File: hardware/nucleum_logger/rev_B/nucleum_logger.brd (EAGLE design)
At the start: 34.9 x 73 mm, 16 parts, among them J1 DM3AT-SF-PEJM5, J2 AA_BAT_PACKSMD, J3 SQUALL_HEADER_BASE, Q1 NX3008PBK, U1 NUCLEUM

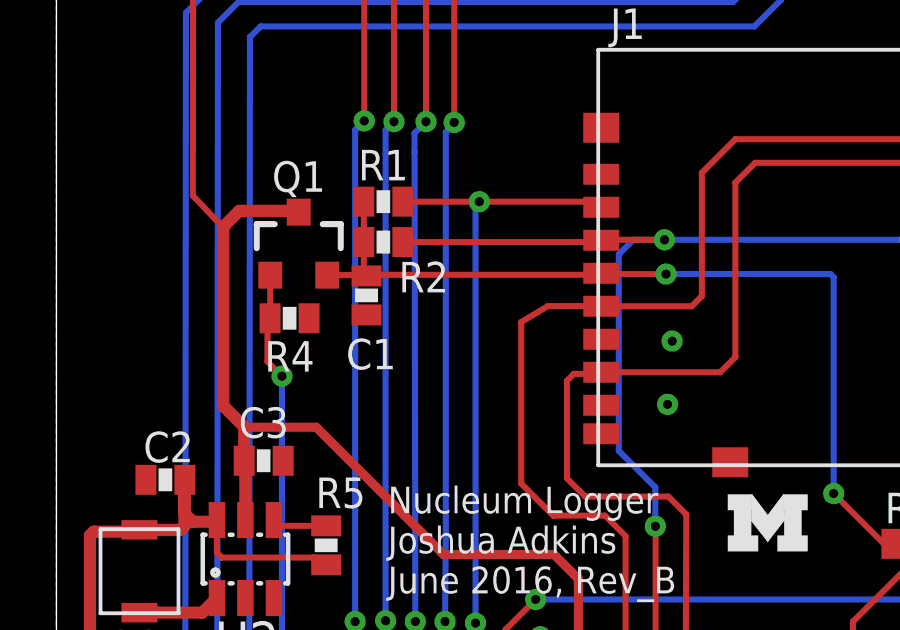
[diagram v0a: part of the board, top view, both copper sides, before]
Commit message: added a rev_B of nucleum logger - we go to production
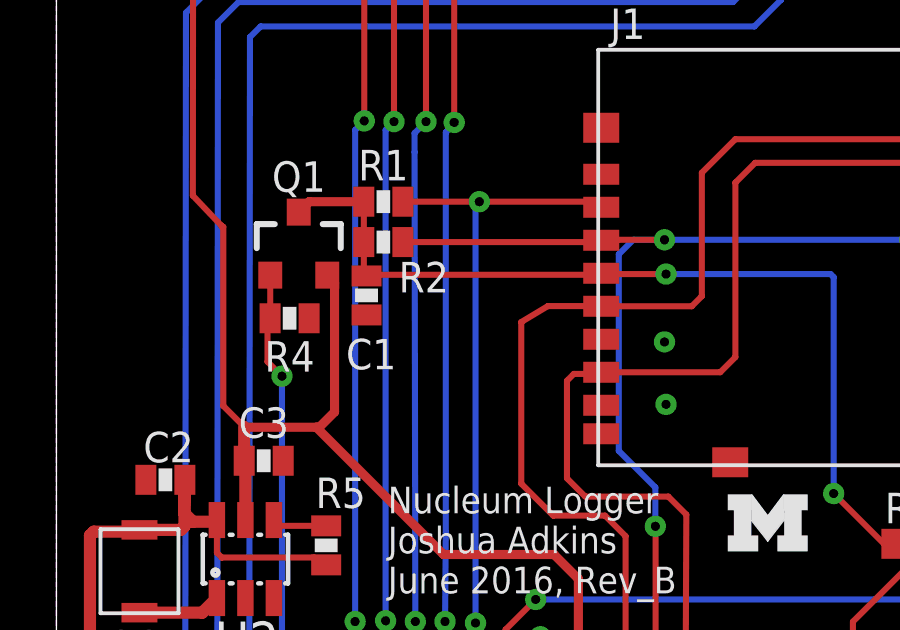
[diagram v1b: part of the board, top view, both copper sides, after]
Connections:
- net VCC: now also Q1.2; no longer Q1.3
- net V_SD: now also Q1.3; no longer Q1.2
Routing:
- net VCC: track 75.0 -> 77.7 mm
- net V_SD: track 30.3 -> 31.3 mm
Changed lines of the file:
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@@
 <layer number="20" name="Dimension" color="15" fill="1" visible="yes" active="yes"/>
 <layer number="21" name="tPlace" color="7" fill="1" visible="yes" active="yes"/>
-<layer number="22" name="bPlace" color="7" fill="1" visible="yes" active="yes"/>
-<layer number="23" name="tOrigins" color="15" fill="1" visible="yes" active="yes"/>
-<layer number="24" name="bOrigins" color="15" fill="1" visible="yes" active="yes"/>
+<layer number="22" name="bPlace" color="7" fill="1" visible="no" active="yes"/>
+<layer number="23" name="tOrigins" color="15" fill="1" visible="no" active="yes"/>
+<layer number="24" name="bOrigins" color="15" fill="1" visible="no" active="yes"/>
 <layer number="25" name="tNames" color="7" fill="1" visible="yes" active="yes"/>
-<layer number="26" name="bNames" color="7" fill="1" visible="yes" active="yes"/>
-<layer number="27" name="tValues" color="7" fill="1" visible="yes" active="yes"/>
-<layer number="28" name="bValues" color="7" fill="1" visible="yes" active="yes"/>
+<layer number="26" name="bNames" color="7" fill="1" visible="no" active="yes"/>
+<layer number="27" name="tValues" color="7" fill="1" visible="no" active="yes"/>
+<layer number="28" name="bValues" color="7" fill="1" visible="no" active="yes"/>
 <layer number="29" name="tStop" color="7" fill="3" visible="no" active="yes"/>
 <layer number="30" name="bStop" color="7" fill="6" visible="no" active="yes"/>
@@
 <layer number="37" name="tTest" color="7" fill="1" visible="no" active="yes"/>
 <layer number="38" name="bTest" color="7" fill="1" visible="no" active="yes"/>
-<layer number="39" name="tKeepout" color="4" fill="11" visible="yes" active="yes"/>
-<layer number="40" name="bKeepout" color="1" fill="11" visible="yes" active="yes"/>
-<layer number="41" name="tRestrict" color="4" fill="10" visible="yes" active="yes"/>
-<layer number="42" name="bRestrict" color="1" fill="10" visible="yes" active="yes"/>
-<layer number="43" name="vRestrict" color="2" fill="10" visible="yes" active="yes"/>
+<layer number="39" name="tKeepout" color="4" fill="11" visible="no" active="yes"/>
+<layer number="40" name="bKeepout" color="1" fill="11" visible="no" active="yes"/>
+<layer number="41" name="tRestrict" color="4" fill="10" visible="no" active="yes"/>
+<layer number="42" name="bRestrict" color="1" fill="10" visible="no" active="yes"/>
+<layer number="43" name="vRestrict" color="2" fill="10" visible="no" active="yes"/>
 <layer number="44" name="Drills" color="7" fill="1" visible="no" active="yes"/>
-<layer number="45" name="Holes" color="7" fill="1" visible="yes" active="yes"/>
+<layer number="45" name="Holes" color="7" fill="1" visible="no" active="yes"/>
 <layer number="46" name="Milling" color="3" fill="1" visible="no" active="yes"/>
 <layer number="47" name="Measures" color="7" fill="1" visible="no" active="yes"/>
-<layer number="48" name="Document" color="7" fill="1" visible="yes" active="yes"/>
-<layer number="49" name="Reference" color="7" fill="1" visible="yes" active="yes"/>
+<layer number="48" name="Document" color="7" fill="1" visible="no" active="yes"/>
+<layer number="49" name="Reference" color="7" fill="1" visible="no" active="yes"/>
 <layer number="50" name="dxf" color="7" fill="1" visible="no" active="no"/>
-<layer number="51" name="tDocu" color="7" fill="1" visible="yes" active="yes"/>
-<layer number="52" name="bDocu" color="7" fill="1" visible="yes" active="yes"/>
+<layer number="51" name="tDocu" color="7" fill="1" visible="no" active="yes"/>
+<layer number="52" name="bDocu" color="7" fill="1" visible="no" active="yes"/>
 <layer number="53" name="tGND_GNDA" color="7" fill="9" visible="no" active="no"/>
 <layer number="54" name="bGND_GNDA" color="1" fill="9" visible="no" active="no"/>
@@
 <layer number="105" name="tPlate" color="7" fill="1" visible="no" active="yes"/>
 <layer number="106" name="bPlate" color="7" fill="1" visible="no" active="yes"/>
-<layer number="107" name="Crop" color="2" fill="1" visible="yes" active="yes"/>
+<layer number="107" name="Crop" color="2" fill="1" visible="no" active="yes"/>
 <layer number="108" name="fp8" color="7" fill="1" visible="no" active="yes"/>
 <layer number="109" name="fp9" color="7" fill="1" visible="no" active="yes"/>
@@
 <layer number="144" name="Drill_legend" color="7" fill="1" visible="no" active="yes"/>
 <layer number="151" name="HeatSink" color="7" fill="1" visible="no" active="yes"/>
-<layer number="199" name="Contour" color="7" fill="1" visible="yes" active="yes"/>
+<layer number="199" name="Contour" color="7" fill="1" visible="no" active="yes"/>
 <layer number="200" name="200bmp" color="1" fill="10" visible="no" active="yes"/>
 <layer number="201" name="201bmp" color="1" fill="10" visible="no" active="yes"/>
@@
 <vertex x="34.8996" y="0"/>
 </polygon>
-<via x="20.5232" y="29.972" extent="1-16" drill="0.3048" diameter="0.6096"/>
-<via x="20.3708" y="27.8638" extent="1-16" drill="0.3048" diameter="0.6096"/>
+<via x="20.2692" y="29.9466" extent="1-16" drill="0.3048" diameter="0.6096"/>
+<via x="20.32" y="27.8638" extent="1-16" drill="0.3048" diameter="0.6096"/>
 <via x="7.7216" y="54.7624" extent="1-16" drill="0.3048" diameter="0.6096"/>
 <contactref element="C1" pad="2"/>
@@
 <contactref element="U2" pad="5"/>
 <contactref element="C3" pad="1"/>
-<contactref element="Q1" pad="3"/>
 <wire x1="6.2992" y1="24.0076" x2="6.2992" y2="25.9438" width="0.4064" layer="1"/>
 <wire x1="6.2992" y1="25.9438" x2="6.2588" y2="25.9842" width="0.4064" layer="1"/>
 <wire x1="6.2588" y1="25.9842" x2="6.2588" y2="27.1168" width="0.4064" layer="1"/>
-<wire x1="6.2588" y1="27.1168" x2="5.5626" y2="27.813" width="0.4064" layer="1"/>
-<wire x1="5.5626" y1="27.813" x2="5.5626" y2="33.782" width="0.4064" layer="1"/>
-<wire x1="5.5626" y1="33.782" x2="6.096" y2="34.3154" width="0.4064" layer="1"/>
-<wire x1="6.096" y1="34.3154" x2="8.0342" y2="34.3154" width="0.4064" layer="1"/>
-<wire x1="8.0342" y1="34.3154" x2="8.0772" y2="34.2724" width="0.4064" layer="1"/>
+<wire x1="6.2588" y1="27.1168" x2="5.5626" y2="27.813" width="0.2032" layer="1"/>
+<wire x1="5.5626" y1="27.813" x2="5.5626" y2="33.782" width="0.2032" layer="1"/>
 <wire x1="5.6896" y1="58.6486" x2="5.0038" y2="58.6486" width="0.2032" layer="1"/>
 <wire x1="5.0038" y1="58.6486" x2="4.572" y2="58.2422" width="0.2032" layer="1"/>
@@
 <wire x1="8.6614" y1="27.1018" x2="6.2738" y2="27.1018" width="0.3048" layer="1"/>
 <wire x1="6.2738" y1="27.1018" x2="6.2588" y2="27.1168" width="0.3048" layer="1"/>
+<contactref element="Q1" pad="2"/>
+<wire x1="9.0272" y1="32.1724" x2="9.271" y2="31.9286" width="0.3048" layer="1"/>
+<wire x1="9.271" y1="31.9286" x2="9.271" y2="27.6098" width="0.3048" layer="1"/>
+<wire x1="9.271" y1="27.6098" x2="8.763" y2="27.1018" width="0.3048" layer="1"/>
+<wire x1="8.763" y1="27.1018" x2="8.6614" y2="27.1018" width="0.3048" layer="1"/>
 </signal>
 <signal name="MISO">
@@
 <contactref element="R3" pad="2"/>
 <contactref element="C1" pad="1"/>
-<contactref element="Q1" pad="2"/>
 <wire x1="10.2466" y1="34.6202" x2="10.2466" y2="33.274" width="0.2032" layer="1"/>
 <wire x1="10.2466" y1="33.274" x2="10.2466" y2="32.2372" width="0.2032" layer="1"/>
 <wire x1="10.2466" y1="32.2372" x2="10.3378" y2="32.146" width="0.2032" layer="1"/>
 <wire x1="10.3752" y1="32.1834" x2="10.3378" y2="32.146" width="0.2032" layer="1"/>
-<wire x1="9.0272" y1="32.1724" x2="10.3114" y2="32.1724" width="0.2032" layer="1"/>
 <wire x1="10.3114" y1="32.1724" x2="10.3378" y2="32.146" width="0.2032" layer="1"/>
 <wire x1="25.908" y1="32.1056" x2="25.908" y2="24.892" width="0.2032" layer="16"/>
@@
 <wire x1="20.32" y1="32.2072" x2="18.7706" y2="32.2072" width="0.2032" layer="1"/>
 <wire x1="18.7706" y1="32.2072" x2="18.1594" y2="32.2342" width="0.2032" layer="1"/>
+<contactref element="Q1" pad="3"/>
+<wire x1="8.0772" y1="34.2724" x2="8.425" y2="34.6202" width="0.3048" layer="1"/>
+<wire x1="8.425" y1="34.6202" x2="10.2466" y2="34.6202" width="0.3048" layer="1"/>
 </signal>
 </signals>
